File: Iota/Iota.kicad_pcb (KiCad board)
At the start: 2 copper layers, 31.8 x 54.6 mm, 25 parts, among them J1 USB_B_Mini, J2 Conn_01x12_Male, J3 Conn_01x12_Male, J4 ICSP, U1 ATmega32U4-AU, Y1 16MHz

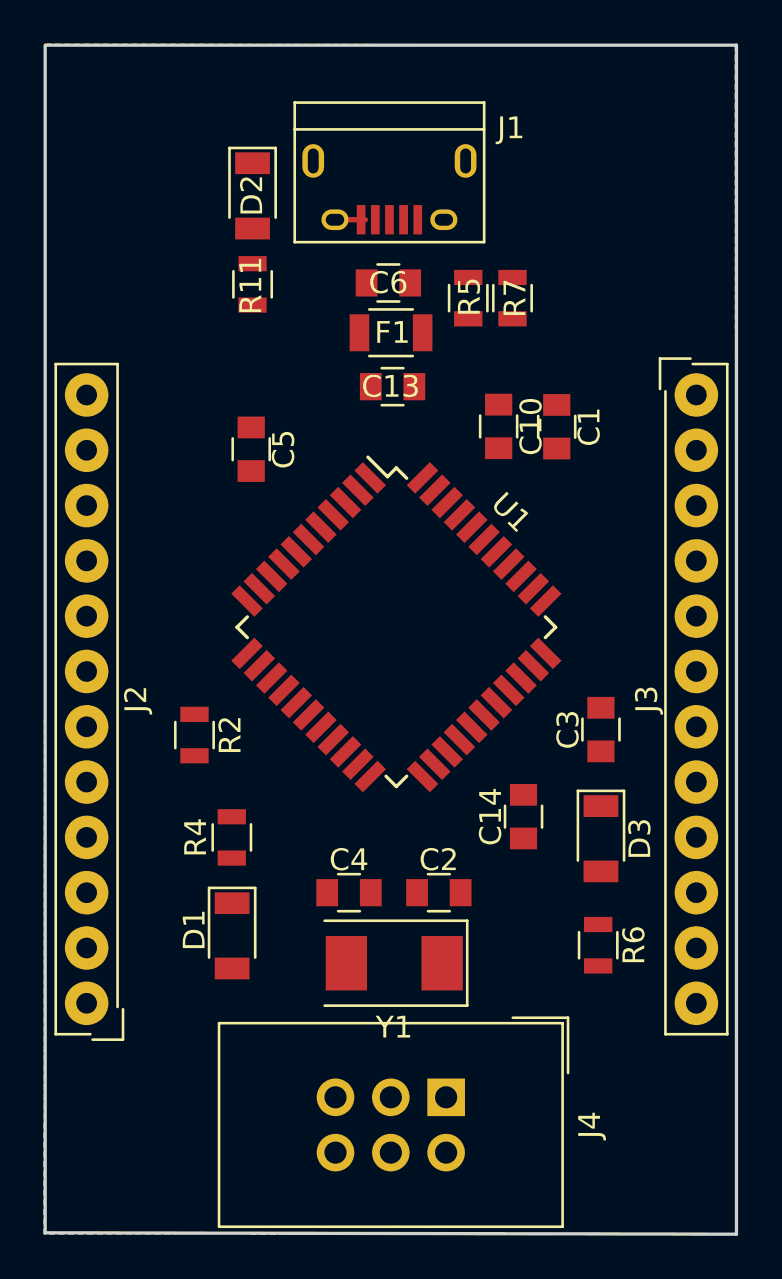
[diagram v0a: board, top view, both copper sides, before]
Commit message: Still faffing around laying out tracks
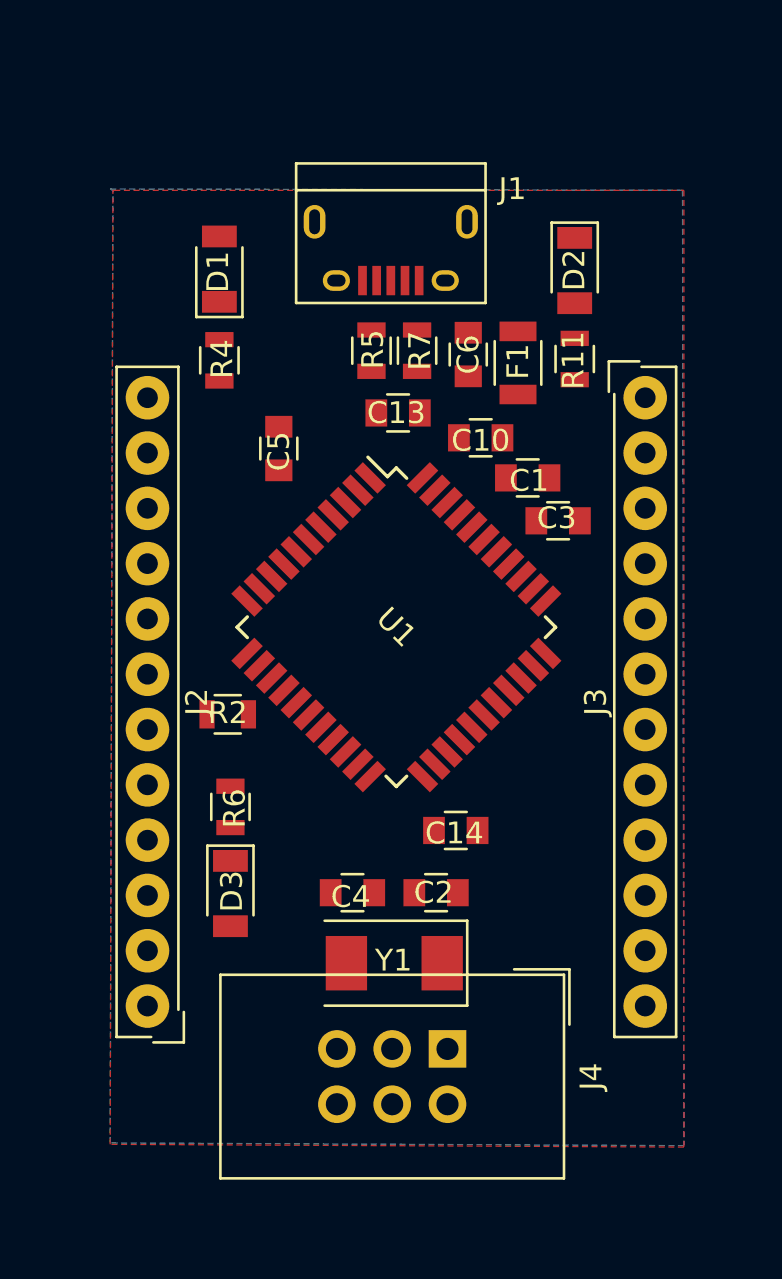
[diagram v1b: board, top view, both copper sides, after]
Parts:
- moved D1 30.6 mm to (125.5, 65.5), turned to 90 degrees
- moved R4 21.9 mm to (125.5, 69.7), turned to 270 degrees
- moved R6 18.0 mm to (126.0, 90.2), turned to 90 degrees
- moved D3 17.2 mm to (126.0, 94.1)
- moved R11 15.2 mm to (141.8, 69.6)
- moved D2 15.2 mm to (141.8, 65.5)
- moved C3 9.79 mm to (141.0, 77.0), turned to 0 degrees
- moved F1 5.99 mm to (139.2, 69.8), turned to 90 degrees
- moved R5 5.06 mm to (132.5, 69.2)
- moved R7 5.00 mm to (134.6, 69.2)
- moved C6 4.92 mm to (136.9, 69.4), turned to 90 degrees
- moved C14 3.18 mm to (136.3, 91.2), turned to 180 degrees
- moved J2 2.80 mm to (122.2, 99.3)
- moved J1 2.79 mm to (133.3, 64.6)
- moved C1 2.70 mm to (139.6, 75.1), turned to 180 degrees
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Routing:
- net GND: track 1.20 -> 0.00 mm
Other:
- board outline removed
